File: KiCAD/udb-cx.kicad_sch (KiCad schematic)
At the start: 15 parts, among them J1 SM04B-SRSS-TB(LF)(SN), J2 USB_C_Receptacle, U1 TPD4E05U06DQAR

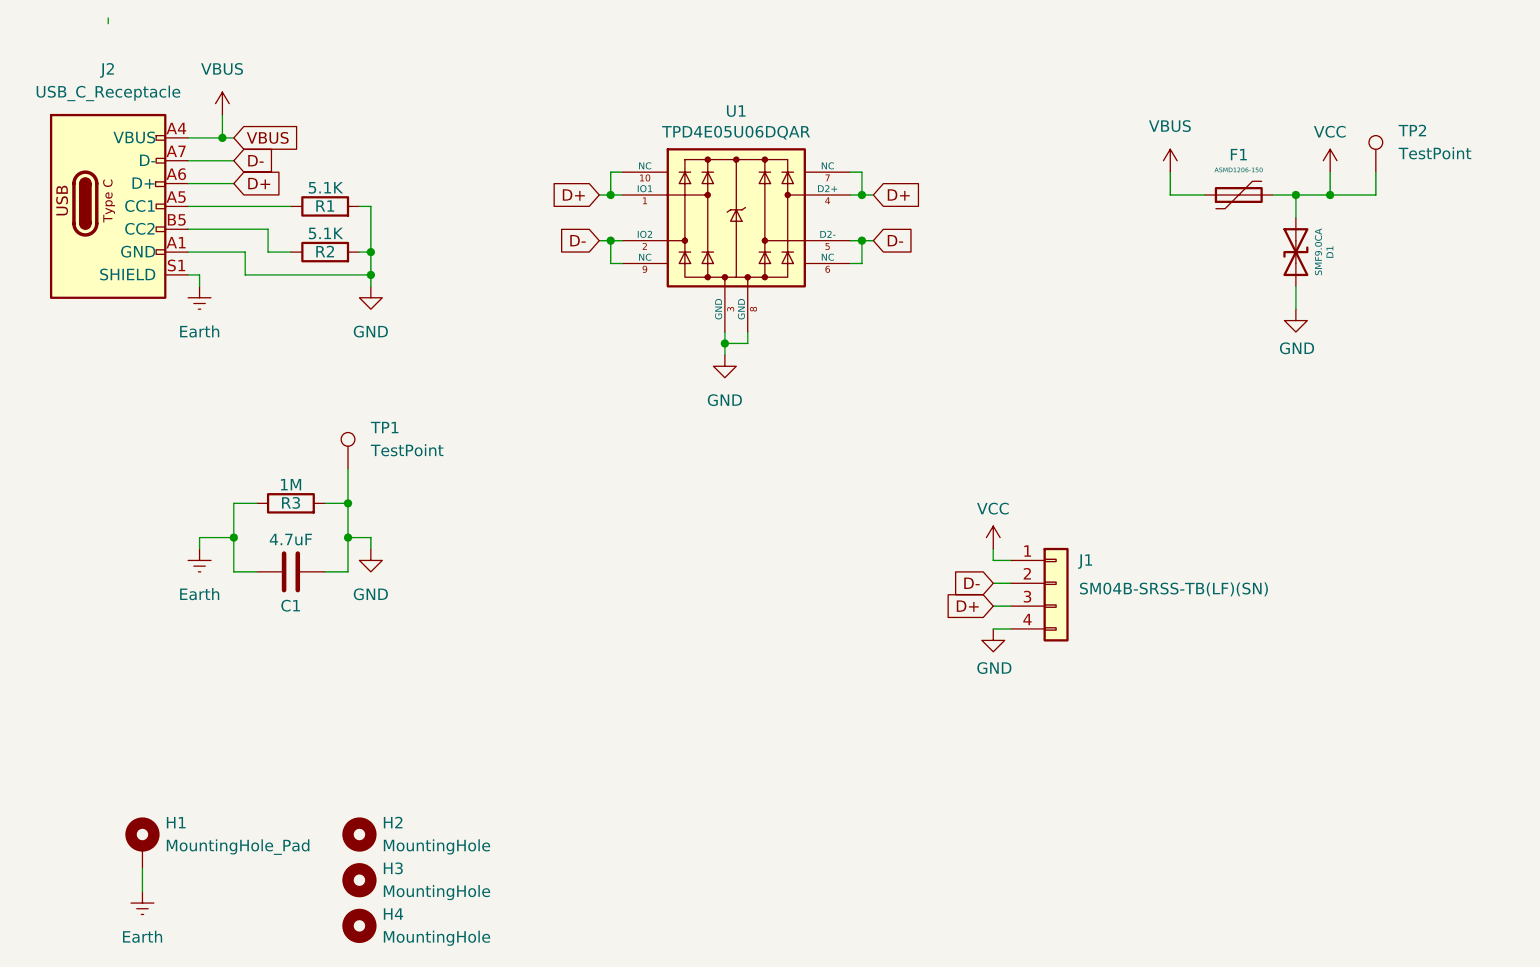
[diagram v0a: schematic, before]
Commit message: .
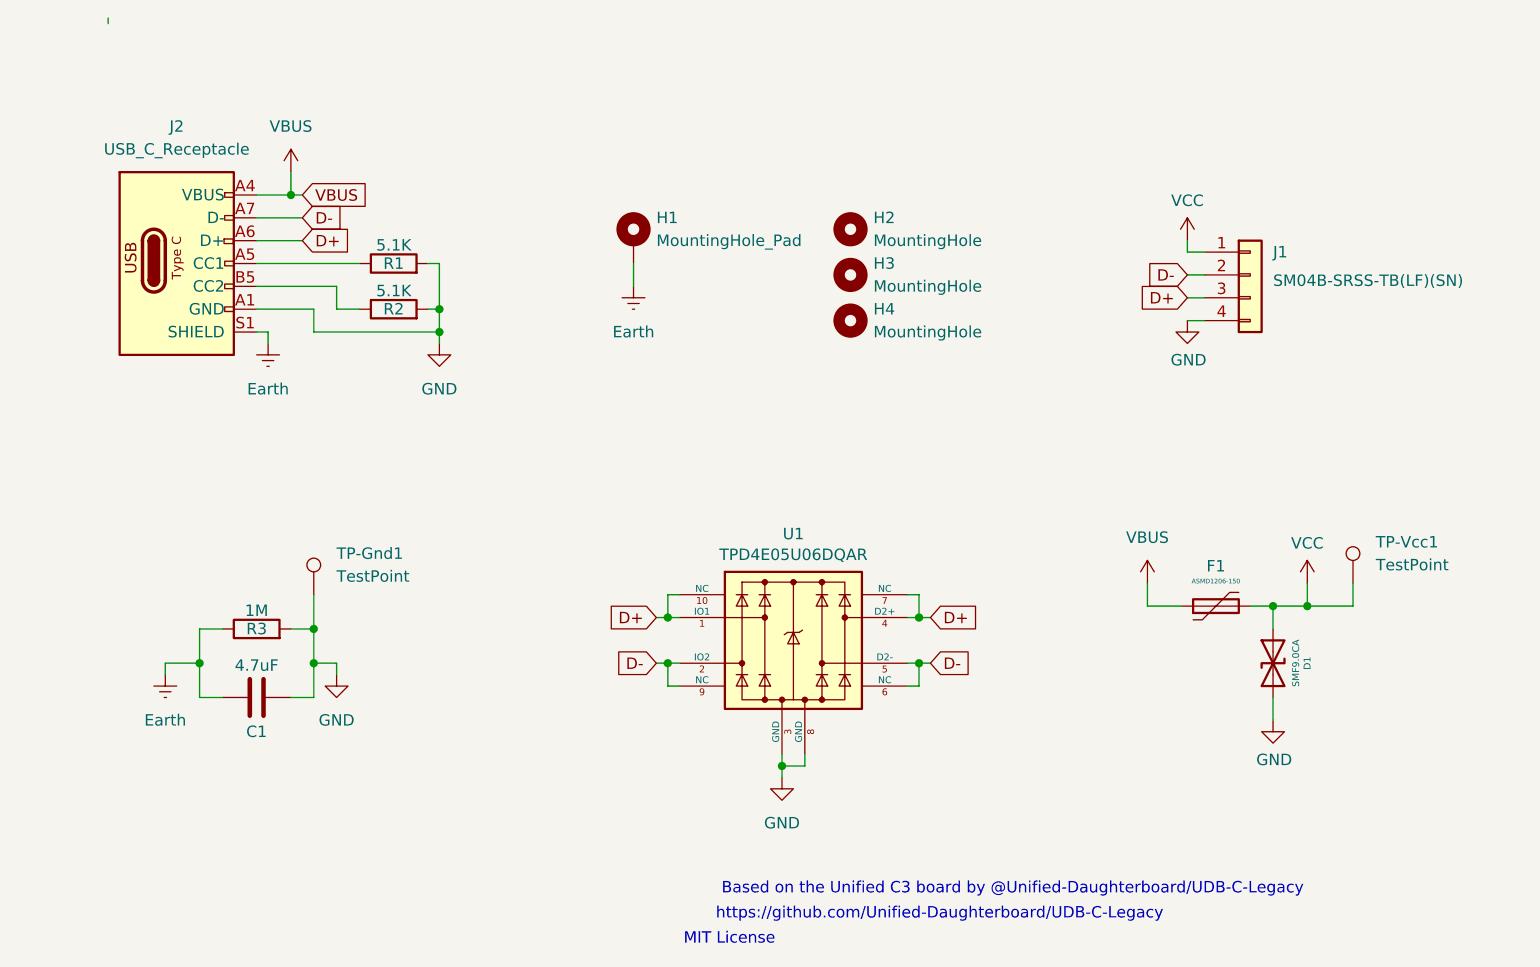
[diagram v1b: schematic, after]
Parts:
- renumbered TP1 to TP-Gnd1, TP2 to TP-Vcc1
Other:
- note added: "Based on the Unified C3 board by @Unified-Daughterboard/UDB-C-Legacy"
- note added: "MIT License"
- note added: "https://github.com/Unified-Daughterboard/UDB-C-Legacy"
- moved on the sheet: C1, D1, F1, H1, H2, H3, H4, J1, J2, R1, R2, R3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

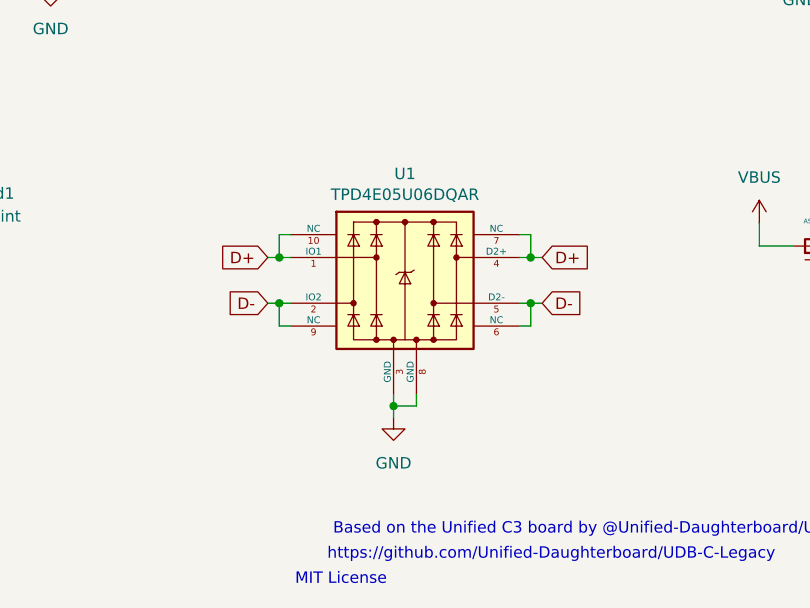
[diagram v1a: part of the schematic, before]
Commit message: .
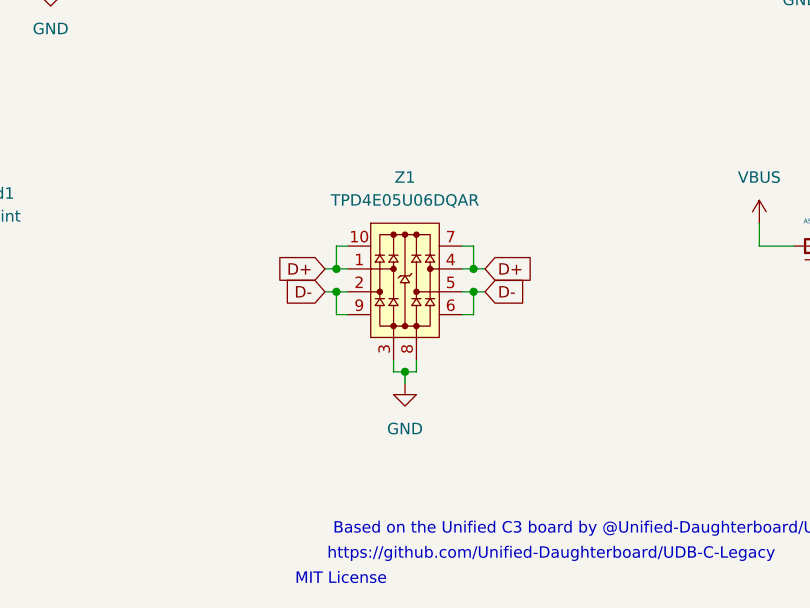
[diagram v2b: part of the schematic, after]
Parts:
- removed U1: TPD4E05U06DQAR, PCM_SparkFun-Semiconductor-Standard:UFDFN-10_2.5x1.0mm_P0.5mm, symbol acheronSymbols:TPD4E05U06DQAR
- added Z1: TPD4E05U06DQAR, PCM_SparkFun-Semiconductor-Standard:UFDFN-10_2.5x1.0mm_P0.5mm, symbol ts-kicad-lib:TPDxE05U06
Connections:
- net D+: now also Z1.1, Z1.10, Z1.4, Z1.7
- net D-: now also Z1.2, Z1.5, Z1.6, Z1.9
- net GND: now also Z1.3, Z1.8
